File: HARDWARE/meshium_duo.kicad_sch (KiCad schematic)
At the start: 0 parts

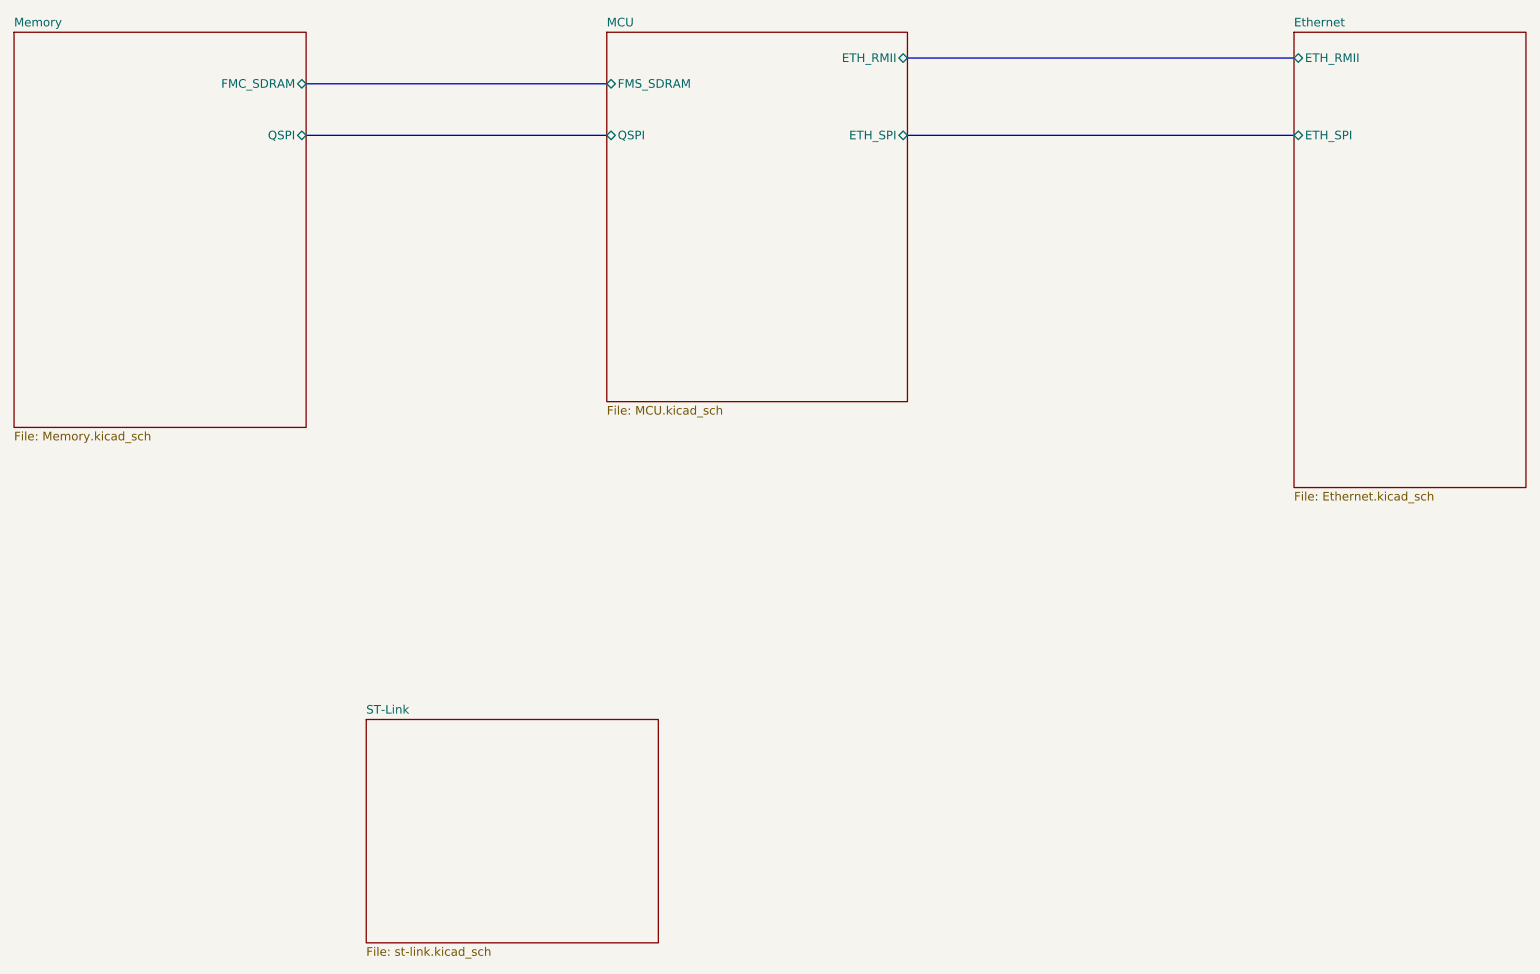
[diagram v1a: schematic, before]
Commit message: schematic capture
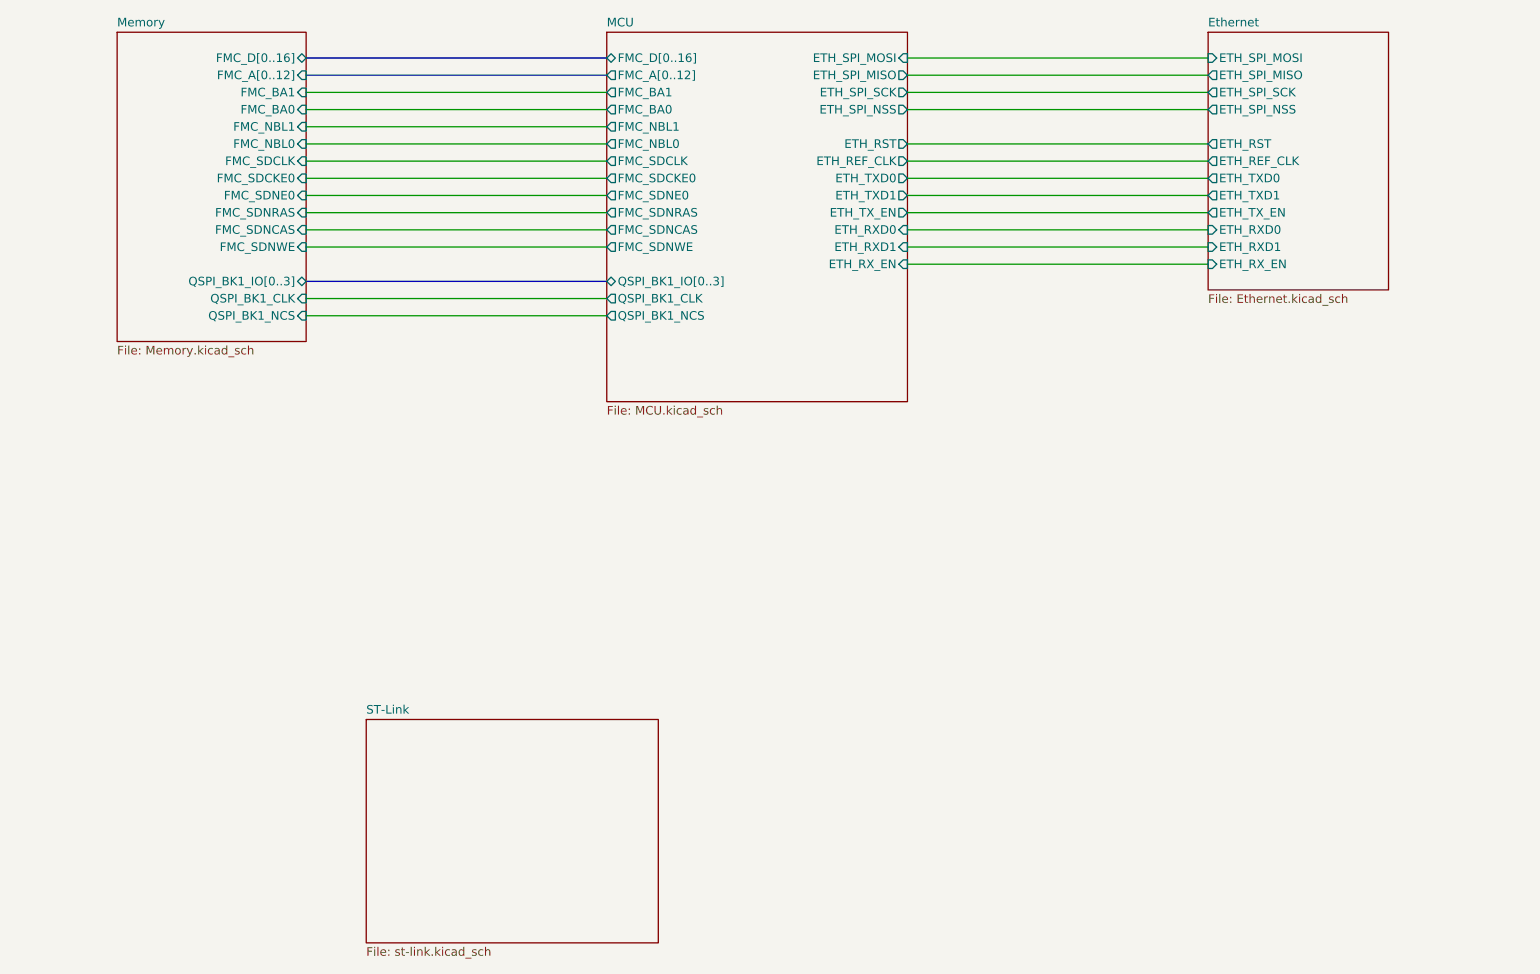
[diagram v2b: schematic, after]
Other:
- sheet Ethernet ports: added ETH_REF_CLK, ETH_RST, ETH_RXD0, ETH_RXD1, ETH_RX_EN, ETH_SPI_MISO, ETH_SPI_MOSI, ETH_SPI_NSS, ETH_SPI_SCK, ETH_TXD0, ETH_TXD1, ETH_TX_EN; removed ETH_RMII, ETH_SPI
- sheet MCU ports: added ETH_REF_CLK, ETH_RST, ETH_RXD0, ETH_RXD1, ETH_RX_EN, ETH_SPI_MISO, ETH_SPI_MOSI, ETH_SPI_NSS, ETH_SPI_SCK, ETH_TXD0, ETH_TXD1, ETH_TX_EN, FMC_A[0..12], FMC_BA0, FMC_BA1, FMC_D[0..16], FMC_NBL0, FMC_NBL1, FMC_SDCKE0, FMC_SDCLK, FMC_SDNCAS, FMC_SDNE0, FMC_SDNRAS, FMC_SDNWE, QSPI_BK1_CLK, QSPI_BK1_IO[0..3], QSPI_BK1_NCS; removed ETH_RMII, ETH_SPI, FMS_SDRAM, QSPI
- sheet Memory ports: added FMC_A[0..12], FMC_BA0, FMC_BA1, FMC_D[0..16], FMC_NBL0, FMC_NBL1, FMC_SDCKE0, FMC_SDCLK, FMC_SDNCAS, FMC_SDNE0, FMC_SDNRAS, FMC_SDNWE, QSPI_BK1_CLK, QSPI_BK1_IO[0..3], QSPI_BK1_NCS; removed FMC_SDRAM, QSPI
